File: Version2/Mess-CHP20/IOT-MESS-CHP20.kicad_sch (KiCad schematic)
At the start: 26 parts, among them J1 Jumper_2, J10 Jumper_2, J2 Jumper, J3 Jumper_2, J4 Jumper, J5 Jumper_2, J7 Conn_01x15_Pin, J8 Conn_01x15_Pin, J9 Jumper_2, K1 Crystal, U1 USB_C_Receptacle_USB2.0_16P, U3 ME6211C33M5

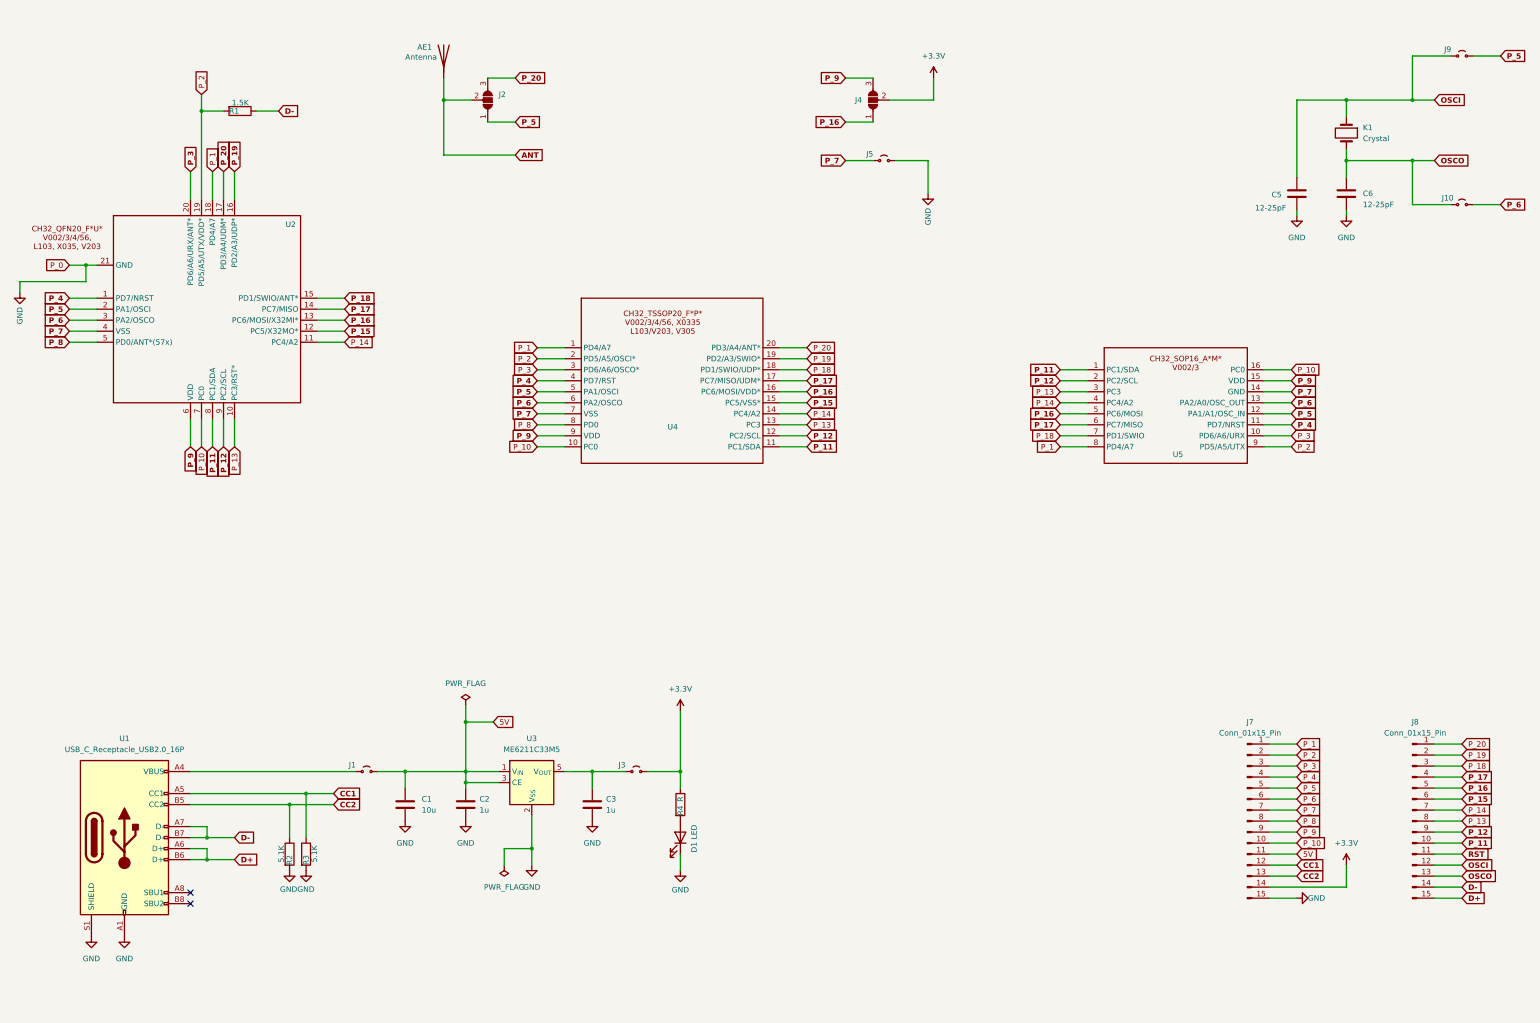
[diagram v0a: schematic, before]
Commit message: updates.
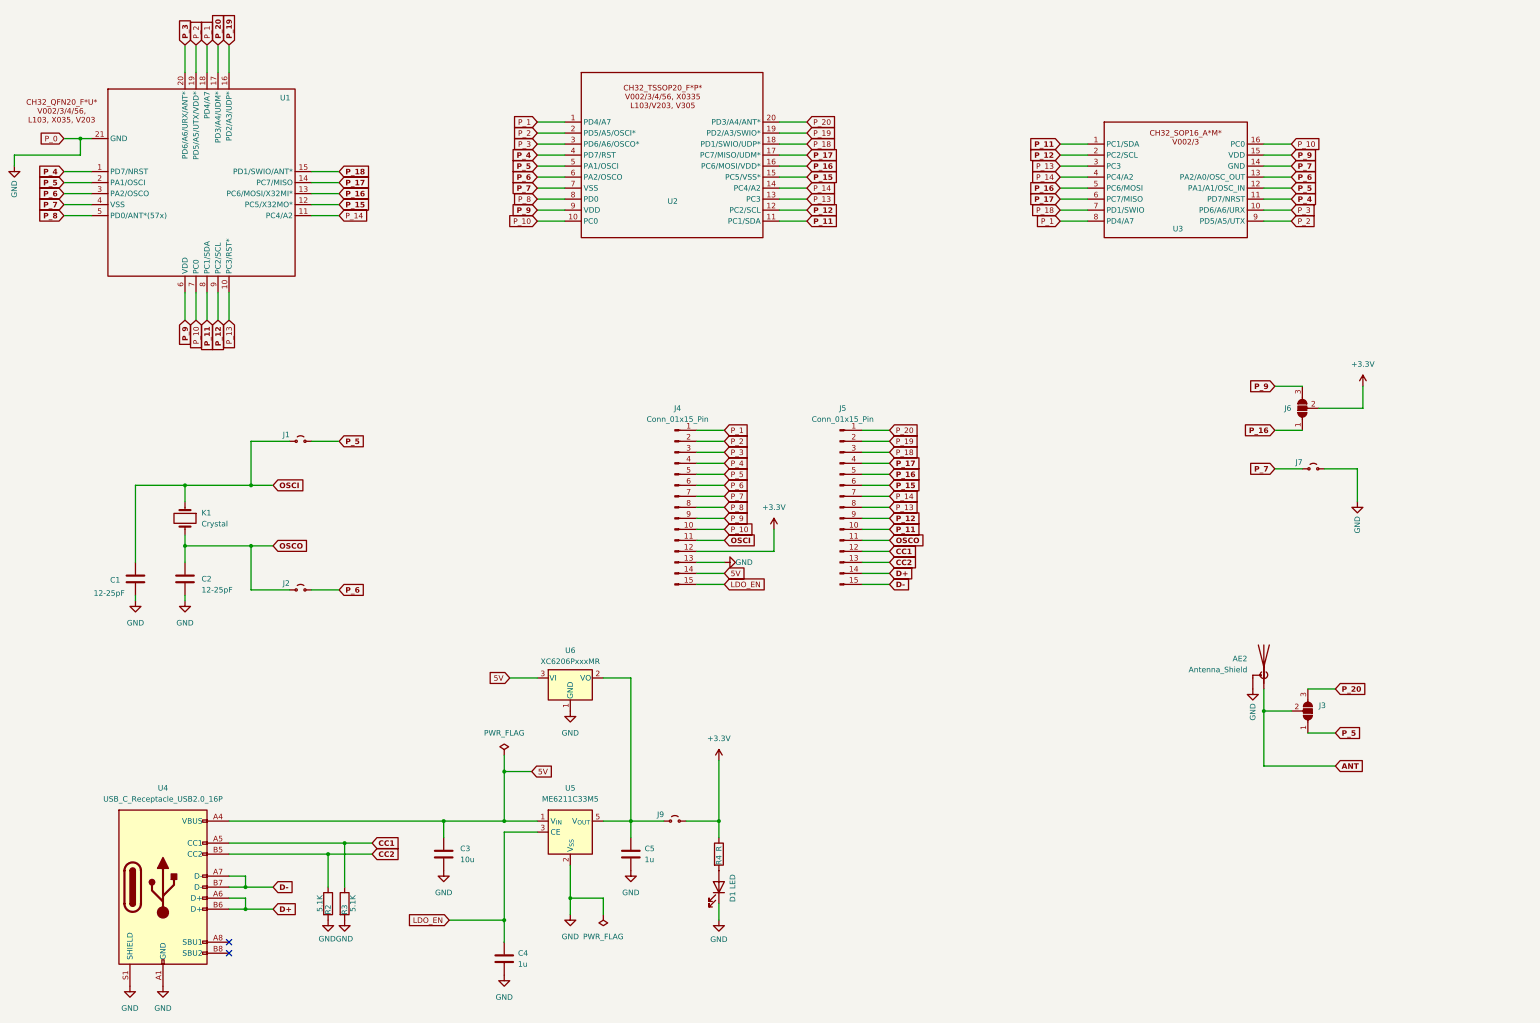
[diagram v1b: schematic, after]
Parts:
- removed AE1: Antenna, RF_Antenna:Texas_SWRA117D_2.4GHz_Right, symbol Device:Antenna
- removed C1: 10u, Capacitor_SMD:C_0603_1608Metric, symbol Device:C
- removed C2: 1u, Capacitor_SMD:C_0603_1608Metric, symbol Device:C
- removed J1, J3: Jumper_2, IOT-Mess-Footprints:Jumpper-triangle, symbol Jumper:Jumper_2_Small_Open
- removed R1: 1.5K, Resistor_SMD:R_0603_1608Metric, symbol Device:R
- removed U1: USB_C_Receptacle_USB2.0_16P, Connector_USB:USB_C_Receptacle_HRO_TYPE-C-31-M-12, symbol Connector:USB_C_Receptacle_USB2.0_16P
- removed U3: ME6211C33M5, Package_TO_SOT_SMD:SOT-23-5, symbol Regulator_Linear:ME6211C33M5
- added AE2: Antenna_Shield, RF_Antenna:Texas_SWRA117D_2.4GHz_Right, symbol Device:Antenna_Shield
- added C3: 10u, Capacitor_SMD:C_0603_1608Metric, symbol Device:C
- added C4: 1u, Capacitor_SMD:C_0603_1608Metric, symbol Device:C
- added J9: Jumper_2, IOT-Mess-Footprints:Jumpper-triangle, symbol Jumper:Jumper_2_Small_Open
- added U4: USB_C_Receptacle_USB2.0_16P, Connector_USB:USB_C_Receptacle_HRO_TYPE-C-31-M-12, symbol Connector:USB_C_Receptacle_USB2.0_16P
- added U5: ME6211C33M5, Package_TO_SOT_SMD:SOT-23-5, symbol Regulator_Linear:ME6211C33M5
- added U6: XC6206PxxxMR, Package_TO_SOT_SMD:SOT-23-3, symbol Regulator_Linear:XC6206PxxxMR
- renumbered C5 to C1, C6 to C2, C3 to C5, J9 to J1, J10 to J2, J2 to J3, J7 to J4, J8 to J5, J4 to J6, J5 to J7, U2 to U1, U4 to U2, U5 to U3
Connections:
- net RST is gone; now on net OSCO: J5.11 (Pin_11)
- net +3.3V: now also J4.12 (Pin_12), J9.2 (B); no longer J4.14 (Pin_14)
- net 5V: now also J4.14 (Pin_14), C3.1, U4.A4 (VBUS), U4.A9 (VBUS), U4.B4 (VBUS), U4.B9 (VBUS), U5.1 (V_{IN}), U6.3 (VI); no longer J4.11 (Pin_11)
- net ANT: now also AE2.1 (A)
- net CC1: now also J5.12 (Pin_12), U4.A5 (CC1); no longer J4.12 (Pin_12)
- net CC2: now also J5.13 (Pin_13), U4.B5 (CC2); no longer J4.13 (Pin_13)
- net D+: now also J5.14 (Pin_14), U4.A6 (D+), U4.B6 (D+); no longer J5.15 (Pin_15)
- net D-: now also J5.15 (Pin_15), U4.A7 (D-), U4.B7 (D-); no longer J5.14 (Pin_14)
- net GND: now also J4.13 (Pin_13), AE2.2 (Shield), C3.2, C4.2, U4.A1 (GND), U4.A12 (GND), U4.B1 (GND), U4.B12 (GND), U4.S1 (SHIELD), U5.2 (V_{SS}), U6.1 (GND); no longer J4.15 (Pin_15)
- net OSCI: now also J4.11 (Pin_11); no longer J5.12 (Pin_12)
- net OSCO: no longer J5.13 (Pin_13)
- net at C5.1: now also J9.1 (A), U5.5 (V_{OUT}), U6.2 (VO)
- new net LDO_EN: C4.1, J4.15 (Pin_15), U5.3 (CE)
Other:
- moved on the sheet: C1, C2, C5, D1, J1, J2, J3, J4, J5, J6, J7, K1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
